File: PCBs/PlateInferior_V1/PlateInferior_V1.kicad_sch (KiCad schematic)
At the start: 3 parts, among them J1 Conn_01x04, J2 Conn_01x04, J3 Conn_02x10_Counter_Clockwise

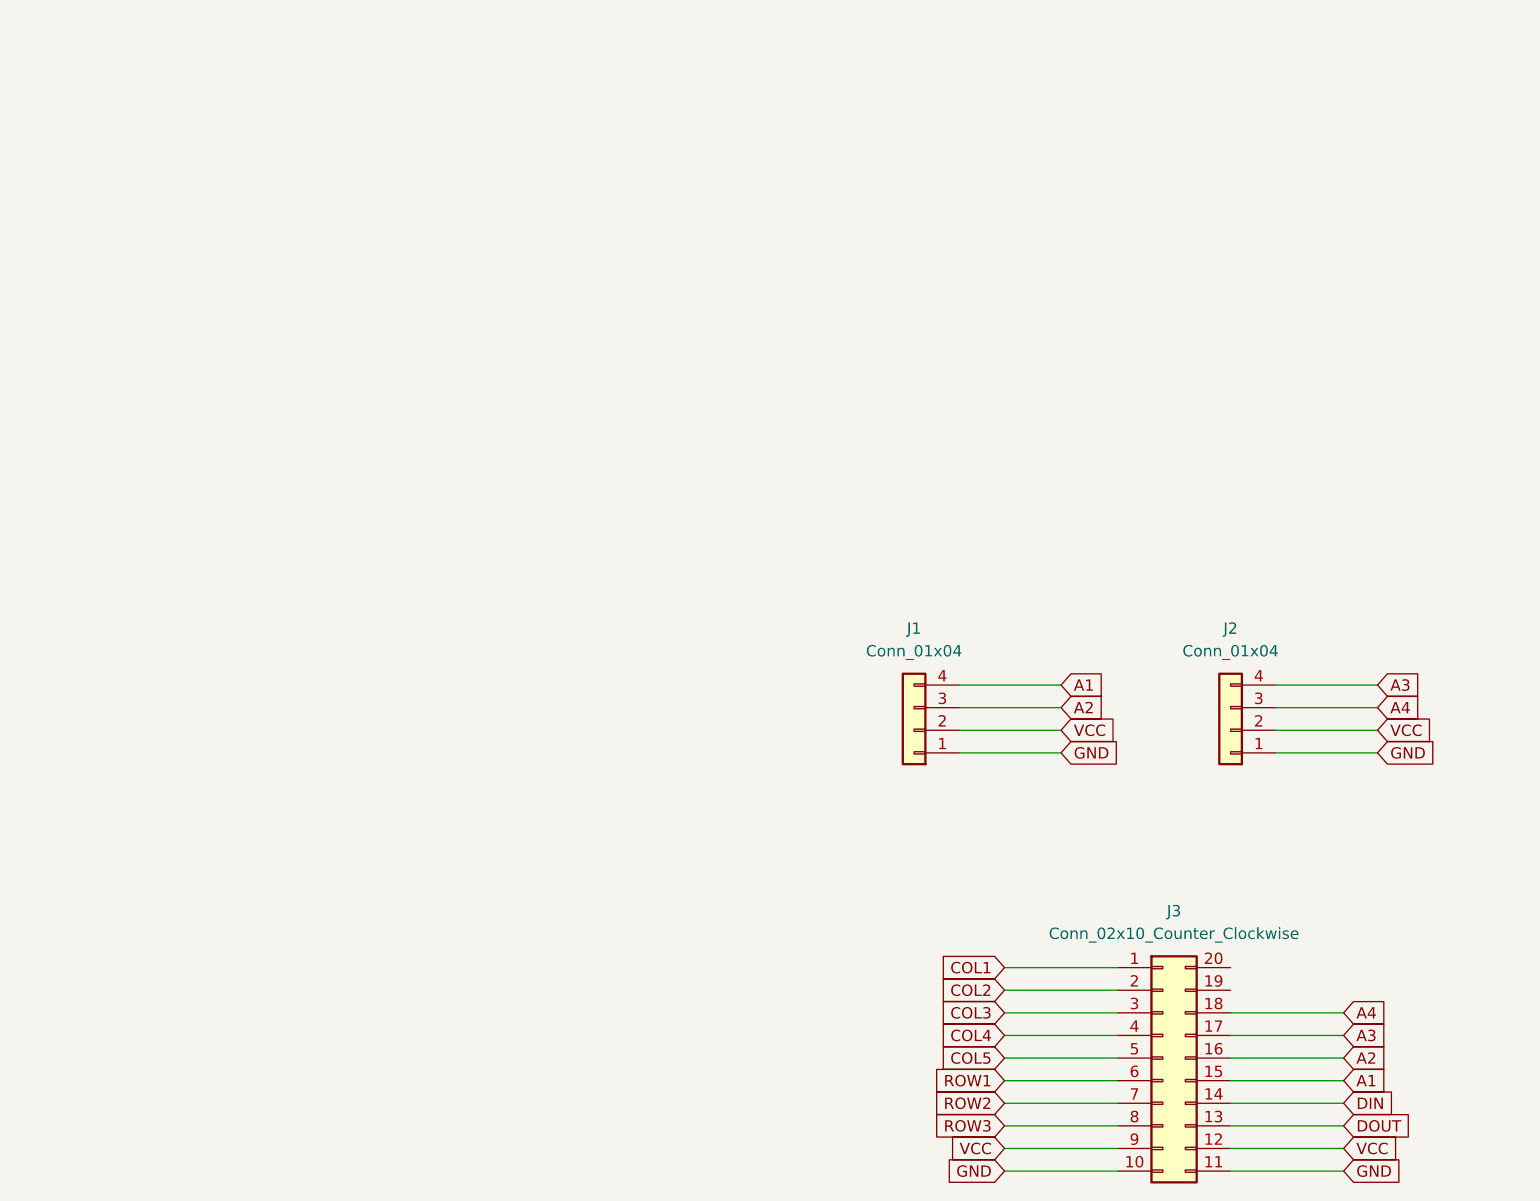
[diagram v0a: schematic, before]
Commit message: Add top PCB
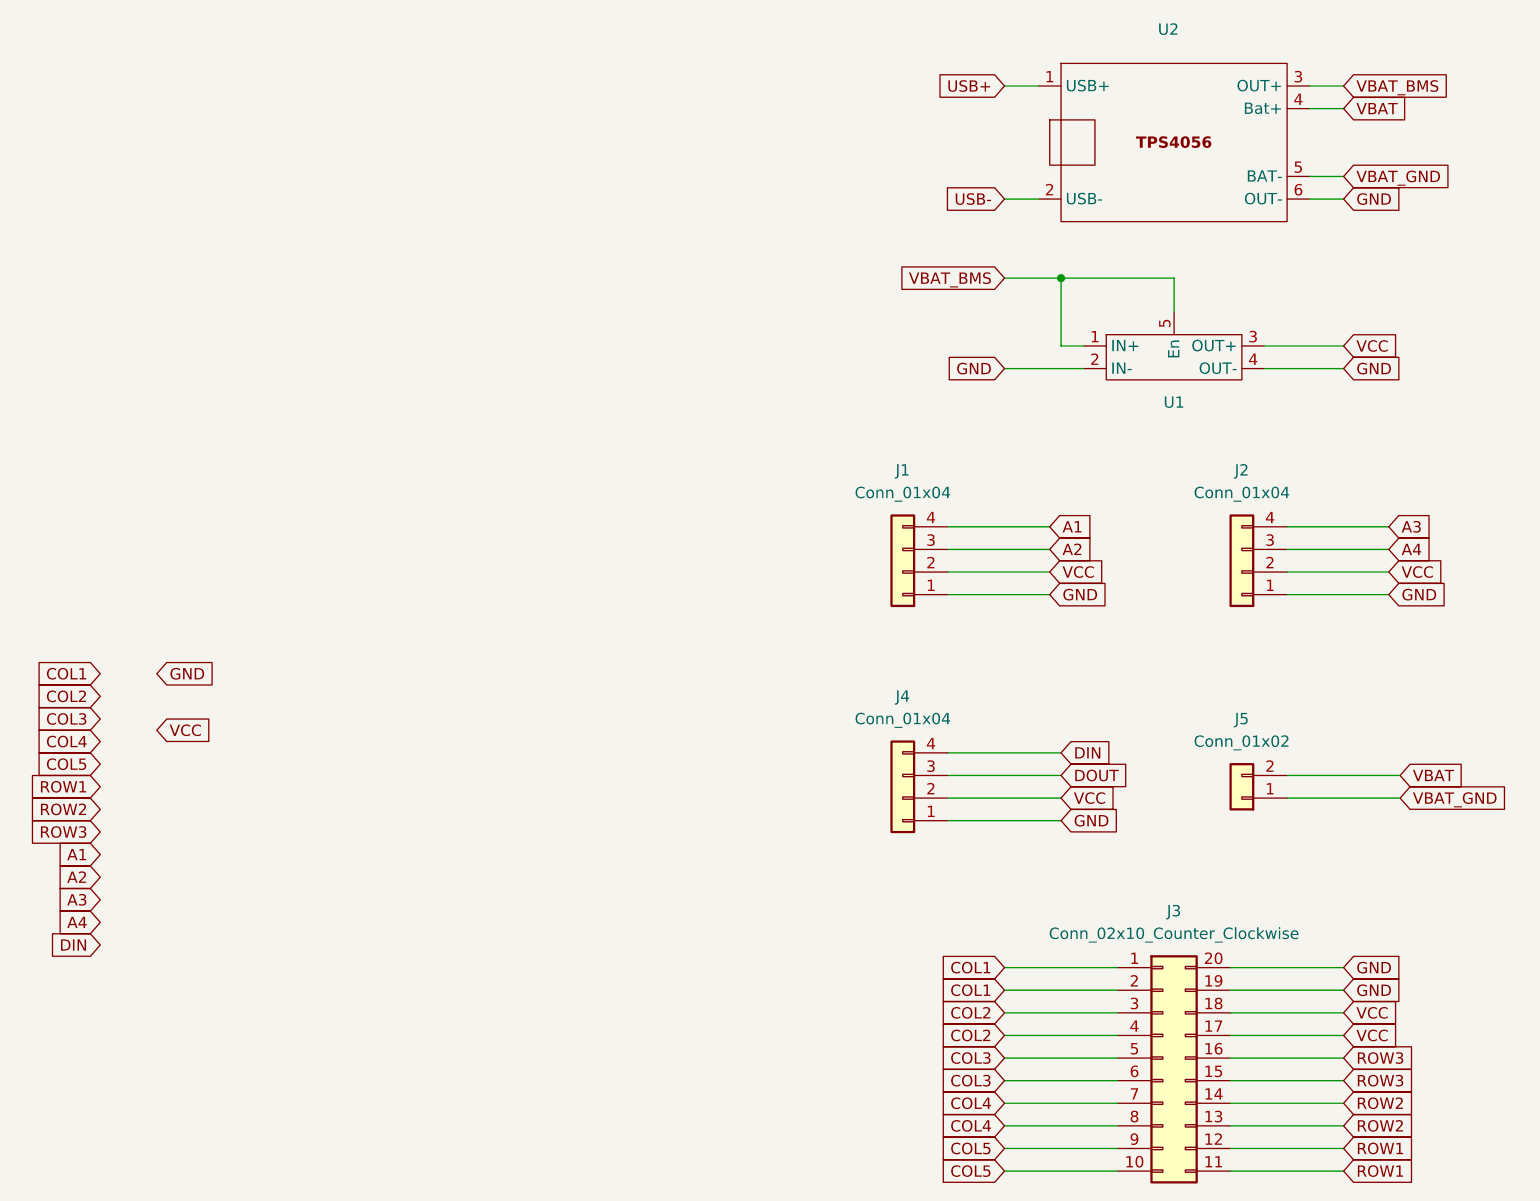
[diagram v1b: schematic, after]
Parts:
- added J4: Conn_01x04, symbol Connector_Generic:Conn_01x04
- added J5: Conn_01x02, symbol Connector_Generic:Conn_01x02
- added U1: ~, dcdc_Var_5W:dcdc_Var_5W, symbol Misc:DCDC_wEnable_1
- added U2: ~, dcdc_Var_5W:TPS4056 Board, symbol Misc:TPS4056_Board
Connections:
- net A1: no longer J3.15 (Pin_15)
- net A2: no longer J3.16 (Pin_16)
- net A3: no longer J3.17 (Pin_17)
- net A4: no longer J3.18 (Pin_18)
- net COL1: now also J3.2 (Pin_2)
- net COL2: now also J3.3 (Pin_3), J3.4 (Pin_4); no longer J3.2 (Pin_2)
- net COL3: now also J3.5 (Pin_5), J3.6 (Pin_6); no longer J3.3 (Pin_3)
- net COL4: now also J3.7 (Pin_7), J3.8 (Pin_8); no longer J3.4 (Pin_4)
- net COL5: now also J3.10 (Pin_10), J3.9 (Pin_9); no longer J3.5 (Pin_5)
- net DIN: now also J4.4 (Pin_4); no longer J3.14 (Pin_14)
- net DOUT: now also J4.3 (Pin_3); no longer J3.13 (Pin_13)
- net GND: now also J3.19 (Pin_19), J3.20 (Pin_20), J4.1 (Pin_1), U1.2 (IN-), U1.4 (OUT-), U2.6 (OUT-); no longer J3.10 (Pin_10), J3.11 (Pin_11)
- net ROW1: now also J3.11 (Pin_11), J3.12 (Pin_12); no longer J3.6 (Pin_6)
- net ROW2: now also J3.13 (Pin_13), J3.14 (Pin_14); no longer J3.7 (Pin_7)
- net ROW3: now also J3.15 (Pin_15), J3.16 (Pin_16); no longer J3.8 (Pin_8)
- net VCC: now also J3.17 (Pin_17), J3.18 (Pin_18), J4.2 (Pin_2), U1.3 (OUT+); no longer J3.12 (Pin_12), J3.9 (Pin_9)
- new net USB+: U2.1 (USB+)
- new net USB-: U2.2 (USB-)
- new net VBAT: J5.2 (Pin_2), U2.4 (Bat+)
- new net VBAT_BMS: U1.1 (IN+), U1.5 (En), U2.3 (OUT+)
- new net VBAT_GND: J5.1 (Pin_1), U2.5 (BAT-)
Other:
- moved on the sheet: J1, J2
